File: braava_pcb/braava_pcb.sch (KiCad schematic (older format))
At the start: 28 parts, among them J1 Conn_01x18, J2 Conn_01x18

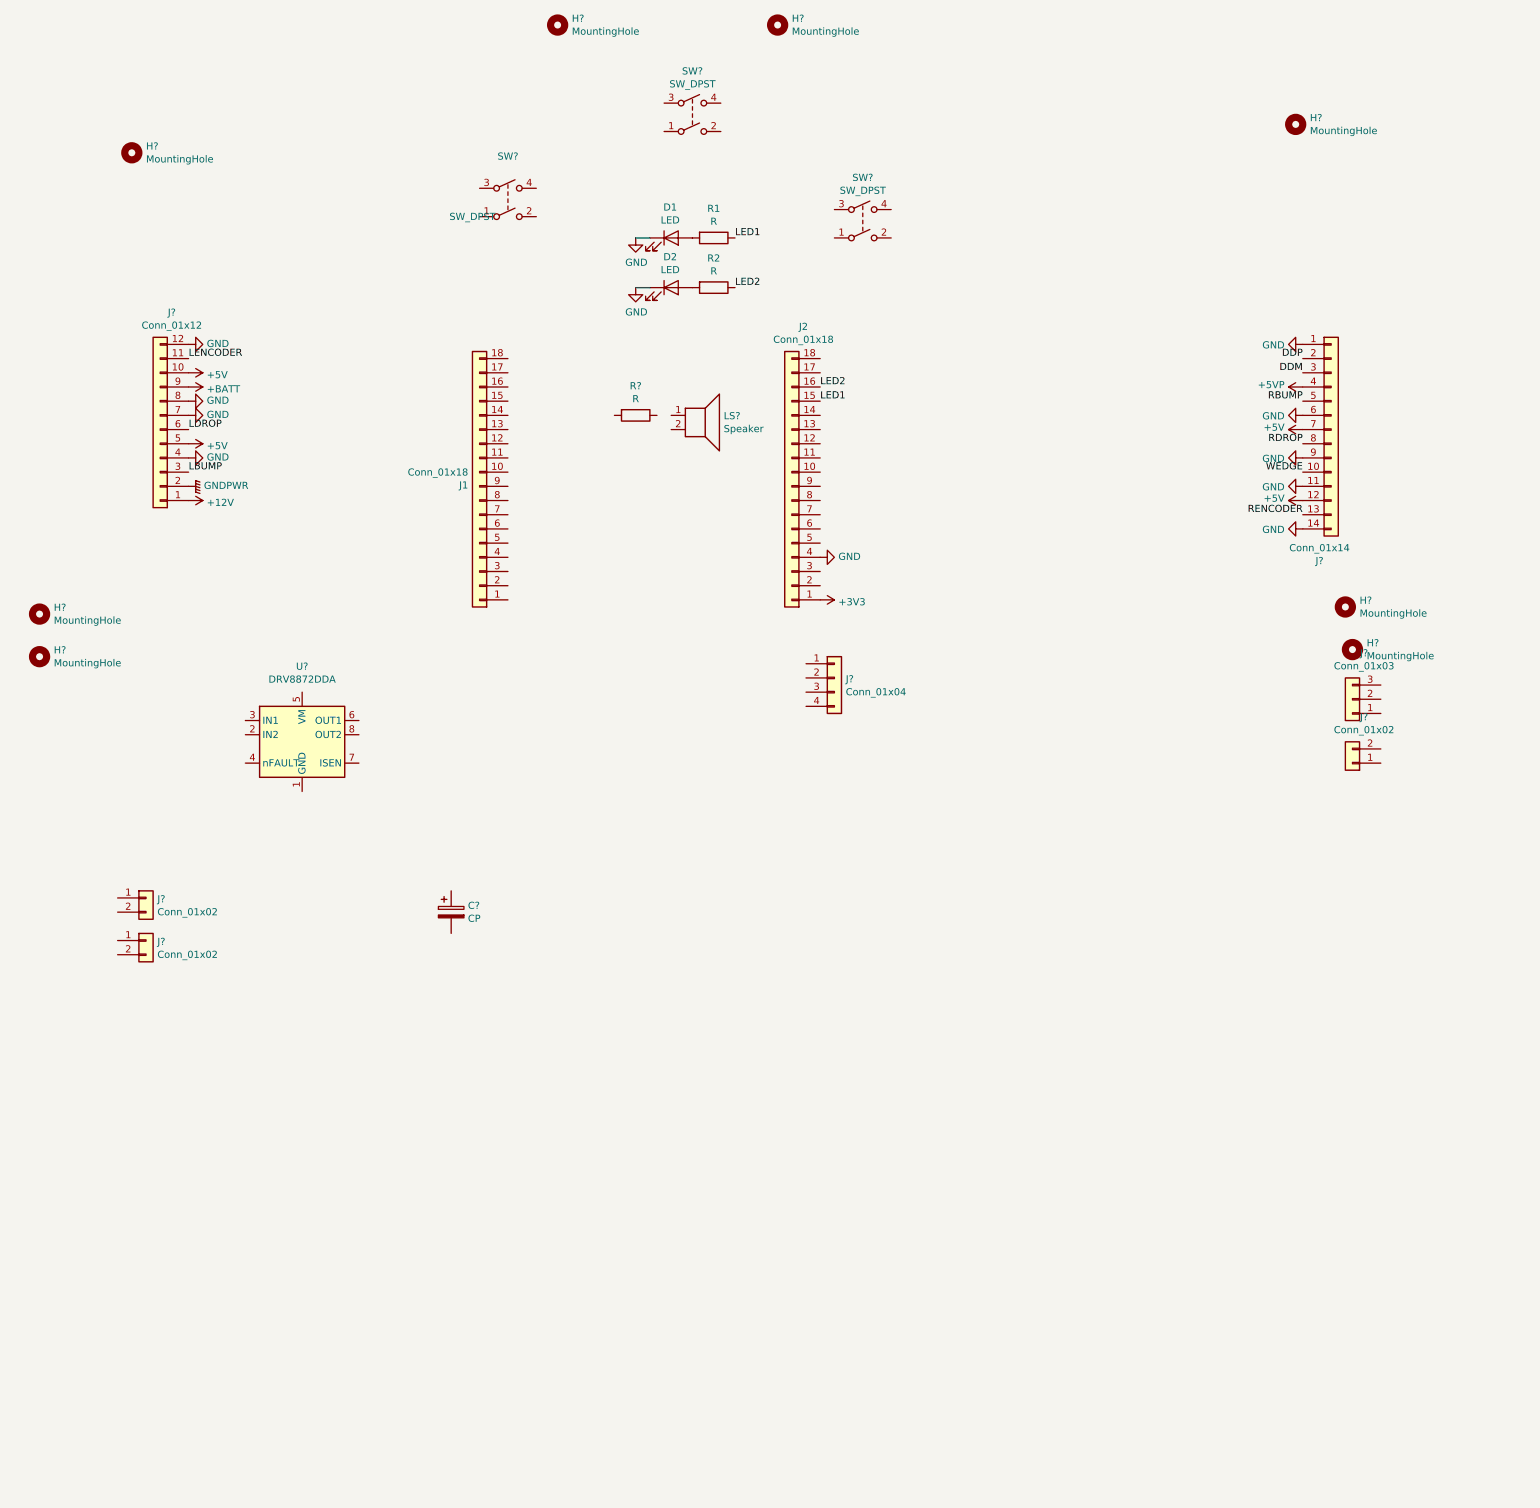
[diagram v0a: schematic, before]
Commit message: Motors, switches near completed
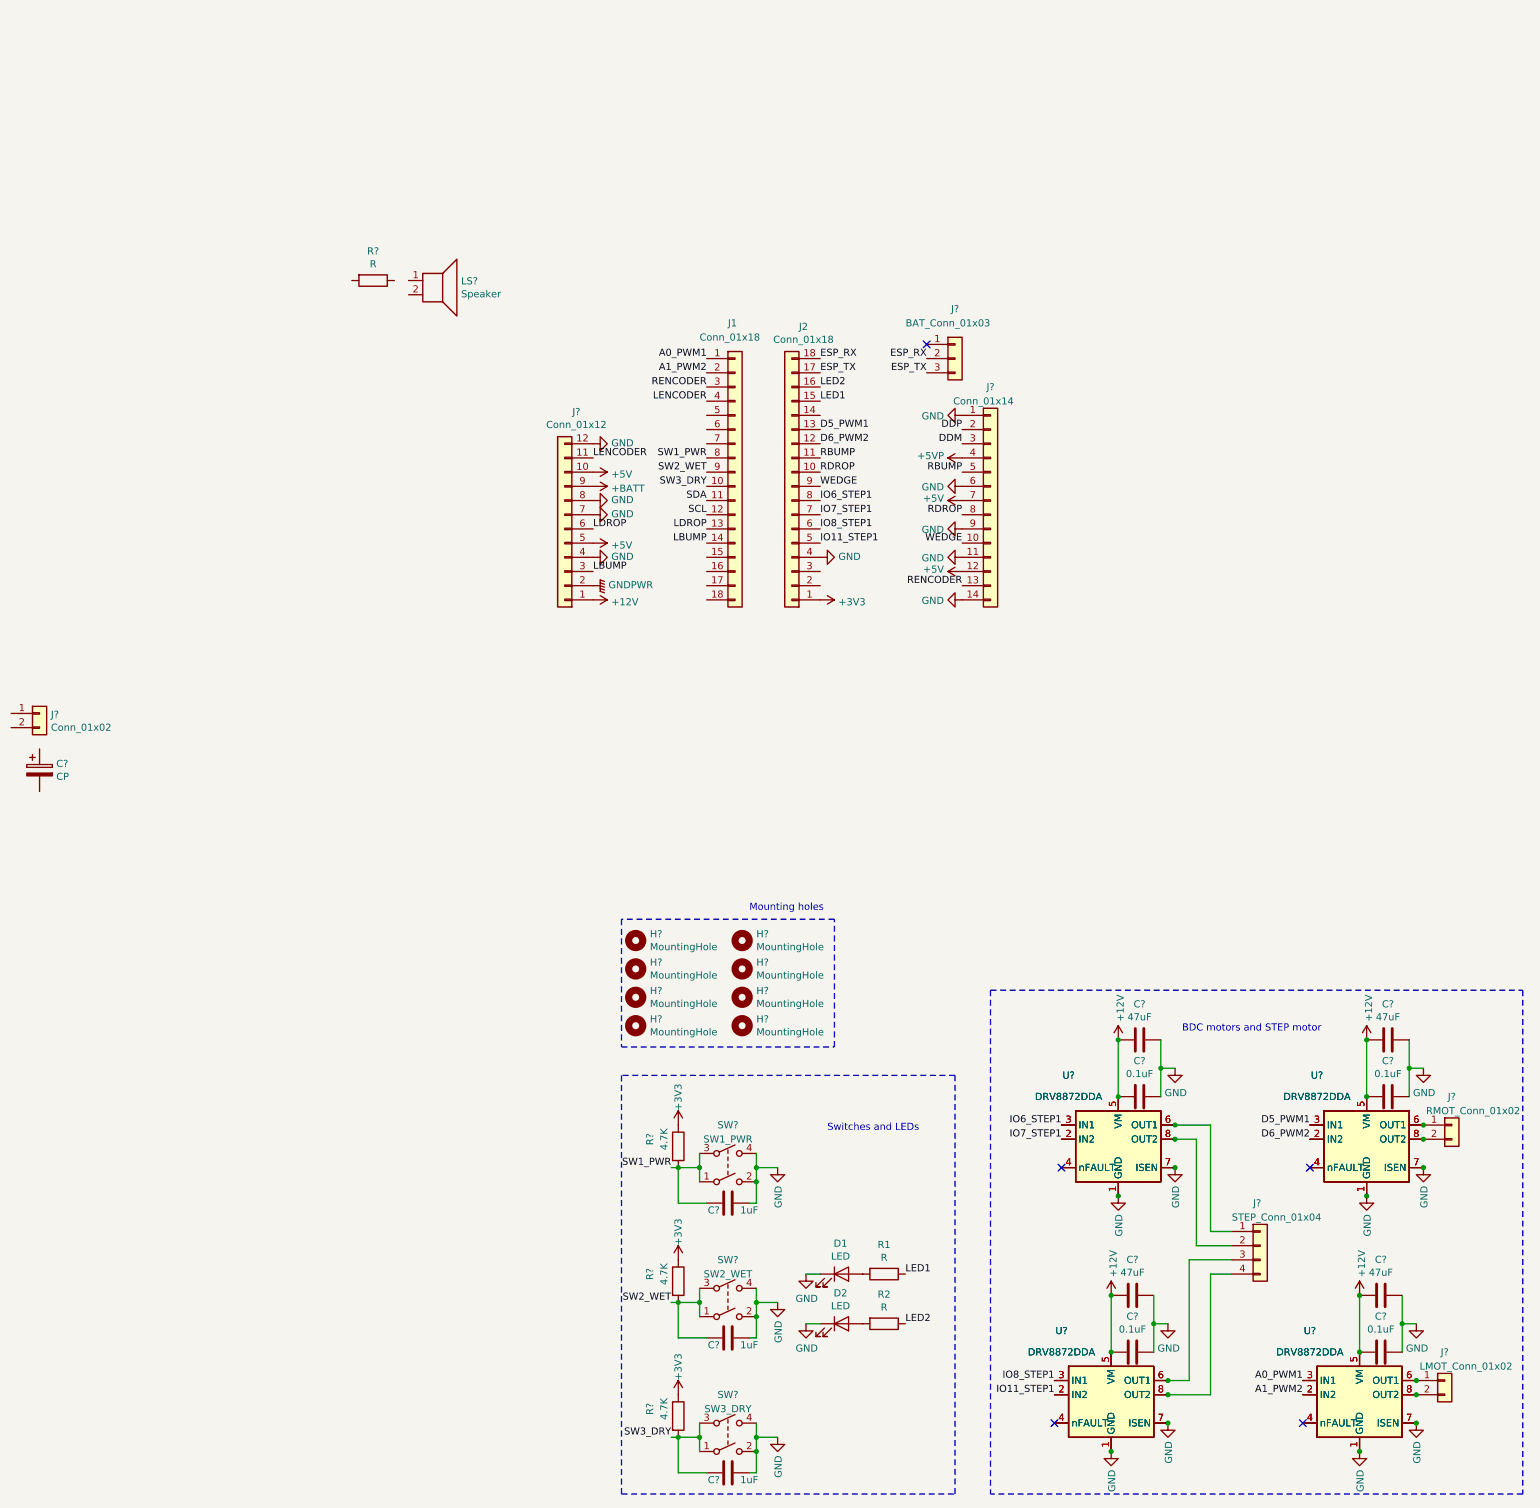
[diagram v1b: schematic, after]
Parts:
- removed J?: Conn_01x02, symbol Connector_Generic:Conn_01x02
- removed SW? (x2): SW_DPST, symbol Switch:SW_DPST
- added C? (x4): 47uF, symbol Device:C
- added C? (x4): 0.1uF, symbol Device:C
- added C? (x3): 1uF, symbol Device:C
- added J?: LMOT_Conn_01x02, symbol Connector_Generic:Conn_01x02
- added R? (x3): 4.7K, Resistor_SMD:R_0603_1608Metric, symbol Device:R
- added SW?: SW2_WET, symbol Switch:SW_DPST
- added SW?: SW3_DRY, symbol Switch:SW_DPST
- added U? (x7): DRV8872DDA, Package_SO:Texas_HTSOP-8-1EP_3.9x4.9mm_P1.27mm_EP2.95x4.9mm_Mask2.4x3.1mm_ThermalVias, symbol Driver_Motor:DRV8872DDA
- J?: value Conn_01x03 -> BAT_Conn_01x03
- J?: value Conn_01x02 -> RMOT_Conn_01x02
- J?: value Conn_01x04 -> STEP_Conn_01x04
- SW?: value SW_DPST -> SW1_PWR
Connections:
- net +12V: now also U?.5 (VM), C?.2, C?.2, C?.2, C?.2, C?.2, C?.2, C?.2, C?.2, U?.5 (VM), U?.5 (VM), U?.5 (VM), U?.5 (VM), U?.5 (VM), U?.5 (VM), U?.5 (VM)
- net +3V3: now also R?.1, R?.1, R?.1
- net GND: now also SW?.2, SW?.4, U?.1 (GND), U?.7 (ISEN), U?.9 (GND), C?.1, C?.1, C?.1, C?.1, C?.1, C?.1, C?.1, C?.1, C?.1, C?.1, C?.1, SW?.2, SW?.2, SW?.4, SW?.4, U?.1 (GND), U?.1 (GND), U?.1 (GND), U?.1 (GND), U?.1 (GND), U?.1 (GND), U?.1 (GND), U?.7 (ISEN), U?.7 (ISEN), U?.7 (ISEN), U?.7 (ISEN), U?.7 (ISEN), U?.7 (ISEN), U?.7 (ISEN), U?.9 (GND), U?.9 (GND), U?.9 (GND), U?.9 (GND), U?.9 (GND), U?.9 (GND), U?.9 (GND)
- net LBUMP: now also J1.14 (Pin_14)
- net LDROP: now also J1.13 (Pin_13)
- net LENCODER: now also J1.4 (Pin_4)
- net RBUMP: now also J2.11 (Pin_11)
- net RDROP: now also J2.10 (Pin_10)
- net RENCODER: now also J1.3 (Pin_3)
- net WEDGE: now also J2.9 (Pin_9)
- net A0_PWM1: now reaches J1.1 (Pin_1)
- net A0_PWM1: now also U?.3 (IN1), U?.3 (IN1)
- net SW3_DRY: now reaches J1.10 (Pin_10)
- net SW3_DRY: now also C?.2, R?.2, SW?.1, SW?.3
- net SDA: now reaches J1.11 (Pin_11)
- net SCL: now reaches J1.12 (Pin_12)
- net A1_PWM2: now reaches J1.2 (Pin_2)
- net A1_PWM2: now also U?.2 (IN2), U?.2 (IN2)
- net SW1_PWR: now reaches J1.8 (Pin_8)
- net SW1_PWR: now also SW?.1, SW?.3, C?.2, R?.2
- net SW2_WET: now reaches J1.9 (Pin_9)
- net SW2_WET: now also C?.2, R?.2, SW?.1, SW?.3
- net D6_PWM2: now reaches J2.12 (Pin_12)
- net D6_PWM2: now also U?.2 (IN2), U?.2 (IN2)
- net D5_PWM1: now reaches J2.13 (Pin_13)
- net D5_PWM1: now also U?.3 (IN1), U?.3 (IN1)
- net ESP_TX: now reaches J2.17 (Pin_17)
- net ESP_TX: now also J?.3 (Pin_3)
- net ESP_RX: now reaches J2.18 (Pin_18)
- net ESP_RX: now also J?.2 (Pin_2)
- net IO11_STEP1: now reaches J2.5 (Pin_5)
- net IO11_STEP1: now also U?.2 (IN2), U?.2 (IN2)
- net IO8_STEP1: now reaches J2.6 (Pin_6)
- net IO8_STEP1: now also U?.3 (IN1), U?.3 (IN1)
- net IO7_STEP1: now reaches J2.7 (Pin_7)
- net IO7_STEP1: now also U?.2 (IN2), U?.2 (IN2)
- net IO6_STEP1: now reaches J2.8 (Pin_8)
- net IO6_STEP1: now also U?.3 (IN1), U?.3 (IN1)
- net at J?.1 (Pin_1): now also U?.6 (OUT1), U?.6 (OUT1) (x2)
- net at J?.2 (Pin_2): now also U?.8 (OUT2), U?.8 (OUT2) (x2)
- net at J?.3 (Pin_3): now also U?.6 (OUT1), U?.6 (OUT1)
- net at J?.4 (Pin_4): now also U?.8 (OUT2), U?.8 (OUT2)
- net at U?.4 (nFAULT): now also U?.4 (nFAULT)
- new net: U?.4 (nFAULT), U?.4 (nFAULT) (x3)
- new net: J?.1 (Pin_1), U?.6 (OUT1), U?.6 (OUT1)
- new net: J?.2 (Pin_2), U?.8 (OUT2), U?.8 (OUT2)
- no-connect marks 0 -> 5
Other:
- note added: "BDC motors and STEP motor"
- note added: "Mounting holes"
- note added: "Switches and LEDs"
- moved on the sheet: C?, D1, D2, H?, J1, J?, LS?, R1, R2, R?, SW?, U?
